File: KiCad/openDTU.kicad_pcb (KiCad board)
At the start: 4 copper layers, 40 x 50 mm, 54 parts, among them J1 USB_C_Receptacle_USB2.0, J2 Conn_Coaxial, J3 Micro_SD_Card, J4 Conn_02x05_Counter_Clockwise, Q1 BC817, Q2 BC817, SW1 SW_Push, SW2 SW_Push, U1 CH340C, U3 ESP32-WROOM-32, U4 nRF24L01P, U5 NCP1117-3.3_SOT223, Y1 16 MHz

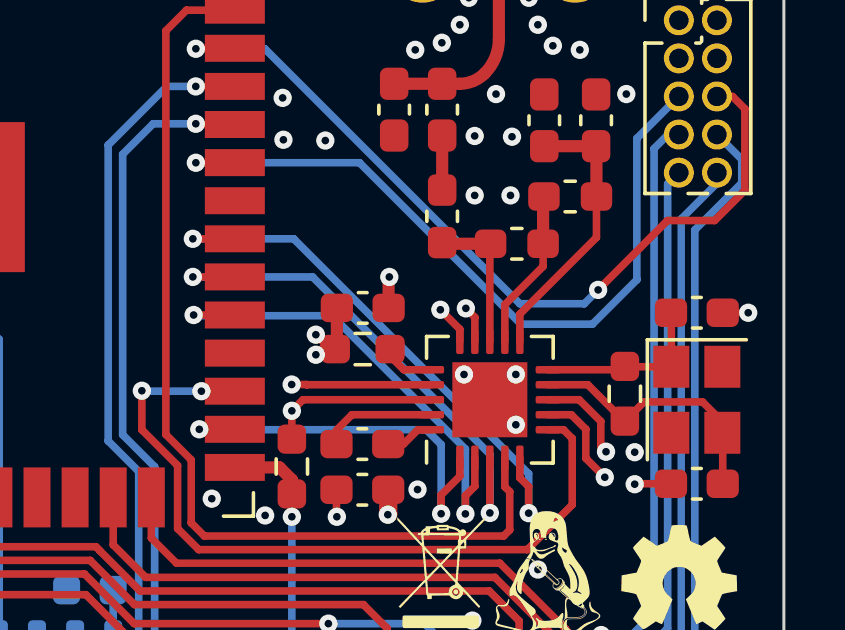
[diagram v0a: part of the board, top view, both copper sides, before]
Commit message: update color of ESP32 wroom module
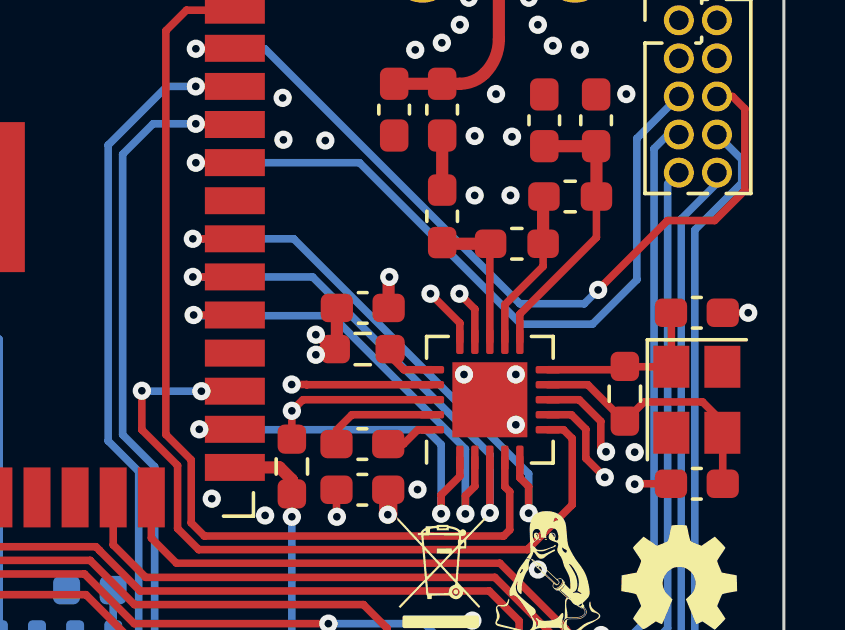
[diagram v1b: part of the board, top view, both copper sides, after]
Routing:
- net +3.3V: track 40.6 -> 41.2 mm
- net GND: track 34.3 -> 34.9 mm
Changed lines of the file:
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@@
       (layer "F.SilkS" (type "Top Silk Screen") (color "White"))
       (layer "F.Paste" (type "Top Solder Paste"))
-      (layer "F.Mask" (type "Top Solder Mask") (color "Blue") (thickness 0.01))
+      (layer "F.Mask" (type "Top Solder Mask") (color "Black") (thickness 0.01))
       (layer "F.Cu" (type "copper") (thickness 0.035))
       (layer "dielectric 1" (type "prepreg") (thickness 0.14) (material "FR4") (epsilon_r 4.5) (loss_tangent 0.02))
@@
       (layer "dielectric 3" (type "prepreg") (thickness 0.14) (material "FR4") (epsilon_r 4.5) (loss_tangent 0.02))
       (layer "B.Cu" (type "copper") (thickness 0.035))
-      (layer "B.Mask" (type "Bottom Solder Mask") (color "Blue") (thickness 0.01))
+      (layer "B.Mask" (type "Bottom Solder Mask") (color "Black") (thickness 0.01))
       (layer "B.Paste" (type "Bottom Solder Paste"))
       (layer "B.SilkS" (type "Bottom Silk Screen") (color "White"))
@@
       )
     )
-    (model "${KICAD6_3DMODEL_DIR}/RF_Module.3dshapes/ESP32-WROOM-32.wrl"
+    (model "${KICAD6_3DMODEL_DIR}/RF_Module.3dshapes/ESP32-WROOM-32.wrl" hide
       (offset (xyz 0 0 0))
       (scale (xyz 1 1 1))
       (rotate (xyz 0 0 0))
     )
+    (model "${KIPRJMOD}/3D_Models/ESP32-WROOM-32.wrl"
+      (offset (xyz 0 3.048 0))
+      (scale (xyz 1 1 1))
+      (rotate (xyz 0 0 -180))
+    )
   )
   (footprint "Inductor_SMD:L_0603_1608Metric_Pad1.05x0.95mm_HandSolder" (layer "F.Cu")
@@
   (segment (start 155.1125 98.9) (end 155.1125 99.4865) (width 0.4064) (layer "F.Cu") (net 1))
   (segment (start 155.575 99.949) (end 155.575 100.875) (width 0.4064) (layer "F.Cu") (net 1))
+  (segment (start 153.7208 86.6648) (end 154.7 87.644) (width 0.254) (layer "F.Cu") (net 1))
   (segment (start 158.8992 92.152156) (end 158.8992 91.1828) (width 0.254) (layer "F.Cu") (net 1))
-  (segment (start 154.05 87.2) (end 154.7 87.85) (width 0.254) (layer "F.Cu") (net 1))
   (segment (start 128.7875 76.8875) (end 128.1 76.8875) (width 0.6096) (layer "F.Cu") (net 1))
   (segment (start 138.95 99.35) (end 139.7 100.1) (width 0.6096) (layer "F.Cu") (net 1))
   (segment (start 129.115 77.215) (end 128.7875 76.8875) (width 0.6096) (layer "F.Cu") (net 1))
+  (segment (start 154.7 87.644) (end 154.7 88.2625) (width 0.254) (layer "F.Cu") (net 1))
   (segment (start 149.1 90.5687) (end 149.4687 90.2) (width 0.254) (layer "F.Cu") (net 1))
   (segment (start 137.7 101.4) (end 137.7 100.35) (width 0.6096) (layer "F.Cu") (net 1))
@@
   (segment (start 149.1 90.5687) (end 149.1 91.5125) (width 0.254) (layer "F.Cu") (net 1))
   (segment (start 150.0892 88.5108) (end 149.9 88.7) (width 0.254) (layer "F.Cu") (net 1))
-  (segment (start 154.7 87.85) (end 154.7 88.2625) (width 0.254) (layer "F.Cu") (net 1))
   (segment (start 158.8992 91.1828) (end 158.4164 90.7) (width 0.254) (layer "F.Cu") (net 1))
   (segment (start 147.2 111.3) (end 147.2 110.6) (width 0.4064) (layer "F.Cu") (net 1))
@@
   (via (at 138.7 101.4) (size 0.8128) (drill 0.4064) (layers "F.Cu" "B.Cu") (net 1))
   (via (at 155.413 99.787) (size 0.6096) (drill 0.254) (layers "F.Cu" "B.Cu") (net 1))
-  (via (at 154.05 87.2) (size 0.6096) (drill 0.254) (layers "F.Cu" "B.Cu") (net 1))
+  (via (at 153.7208 86.6648) (size 0.6096) (drill 0.254) (layers "F.Cu" "B.Cu") (net 1))
   (segment (start 146.015 91.185) (end 147.2 91.185) (width 0.254) (layer "F.Cu") (net 2))
   (segment (start 154.7 92.75) (end 154.7 92.1375) (width 0.254) (layer "F.Cu") (net 2))
@@
   (segment (start 135.1026 106.1974) (end 135.8526 106.1974) (width 0.4064) (layer "F.Cu") (net 8))
   (segment (start 164.3126 87.3) (end 163.4625 87.3) (width 0.254) (layer "F.Cu") (net 8))
+  (segment (start 155.2 87.1788) (end 155.2 88.2625) (width 0.254) (layer "F.Cu") (net 8))
   (segment (start 152.325 87.1392) (end 152.325 86.1302) (width 0.4064) (layer "F.Cu") (net 8))
   (segment (start 153.375 100.875) (end 153.375 99.8122) (width 0.4064) (layer "F.Cu") (net 8))
   (segment (start 132.985 94.7834) (end 132.9944 94.7928) (width 0.6096) (layer "F.Cu") (net 8))
   (segment (start 152.824 91.676) (end 152.3125 91.676) (width 0.254) (layer "F.Cu") (net 8))
-  (segment (start 154.9 87.153603) (end 155.2 87.453603) (width 0.254) (layer "F.Cu") (net 8))
   (segment (start 152.3125 94.0167) (end 152.2984 94.0308) (width 0.6096) (layer "F.Cu") (net 8))
   (segment (start 161.7375 93) (end 160.5428 93) (width 0.254) (layer "F.Cu") (net 8))
@@
   (segment (start 145.5807 104.3807) (end 144.0848 104.3807) (width 0.6096) (layer "F.Cu") (net 8))
   (segment (start 153.3 91.2) (end 152.824 91.676) (width 0.254) (layer "F.Cu") (net 8))
+  (segment (start 154.686 86.6648) (end 155.2 87.1788) (width 0.254) (layer "F.Cu") (net 8))
   (segment (start 159.572422 91.932584) (end 159.398 91.758162) (width 0.254) (layer "F.Cu") (net 8))
-  (segment (start 155.2 87.453603) (end 155.2 88.2625) (width 0.254) (layer "F.Cu") (net 8))
   (segment (start 142.445 110.62) (end 143.02 111.195) (width 0.4064) (layer "F.Cu") (net 8))
   (segment (start 146.7772 105.0299) (end 146.2299 105.0299) (width 0.6096) (layer "F.Cu") (net 8))
@@
   (via (at 137.6934 89.5096) (size 0.6096) (drill 0.254) (layers "F.Cu" "B.Cu") (free) (net 8))
   (via (at 130.5306 109.347) (size 0.6096) (drill 0.254) (layers "F.Cu" "B.Cu") (free) (net 8))
-  (via (at 154.9 87.153603) (size 0.6096) (drill 0.254) (layers "F.Cu" "B.Cu") (net 8))
+  (via (at 154.686 86.6648) (size 0.6096) (drill 0.254) (layers "F.Cu" "B.Cu") (net 8))
   (via (at 149.352 100.838) (size 0.6096) (drill 0.254) (layers "F.Cu" "B.Cu") (free) (net 8))
   (via (at 150.2664 99.7204) (size 0.6096) (drill 0.254) (layers "F.Cu" "B.Cu") (free) (net 8))
